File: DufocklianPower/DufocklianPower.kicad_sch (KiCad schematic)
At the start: 84 parts, among them J1 Conn_Receptacle_3P_Protected, J2 ST7796S, Q1 NMOS, Q2 NMOS, SW1 RST, SW2 BOOT, T1 Transformer_1P_1S, U2 LM5164DDA, U3 OPA388, U4 AD5282, U5 MCP4725, U6 ESP32-S3-WROOM-1, U7 INA228

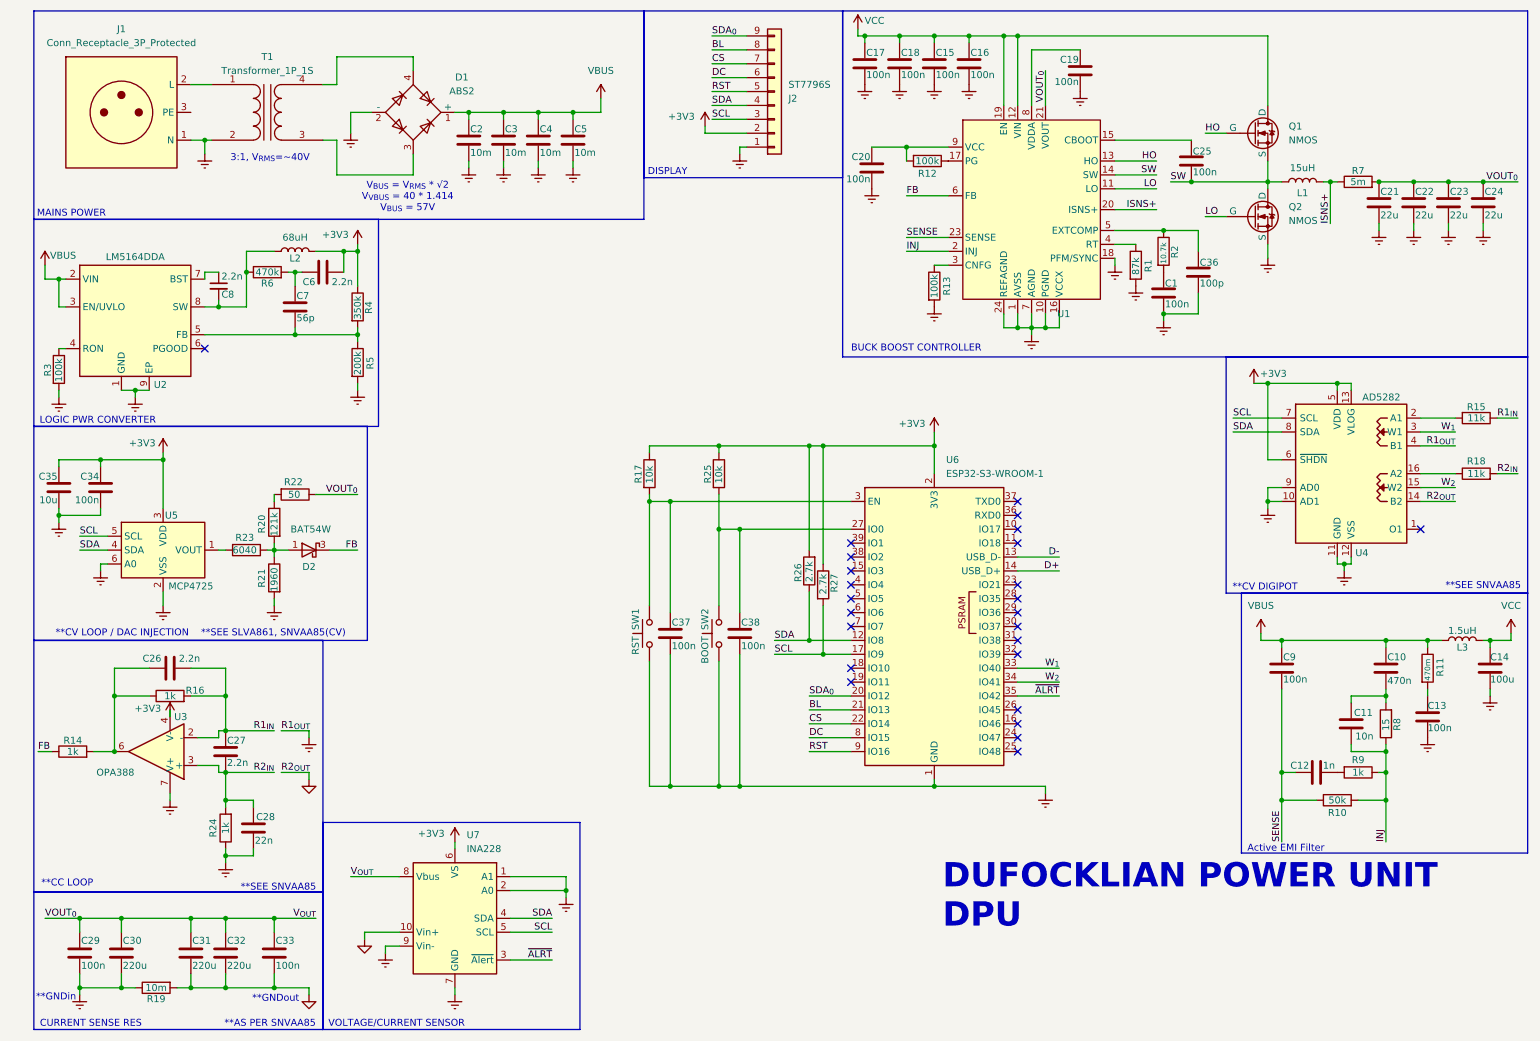
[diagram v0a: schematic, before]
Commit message: finish pcb
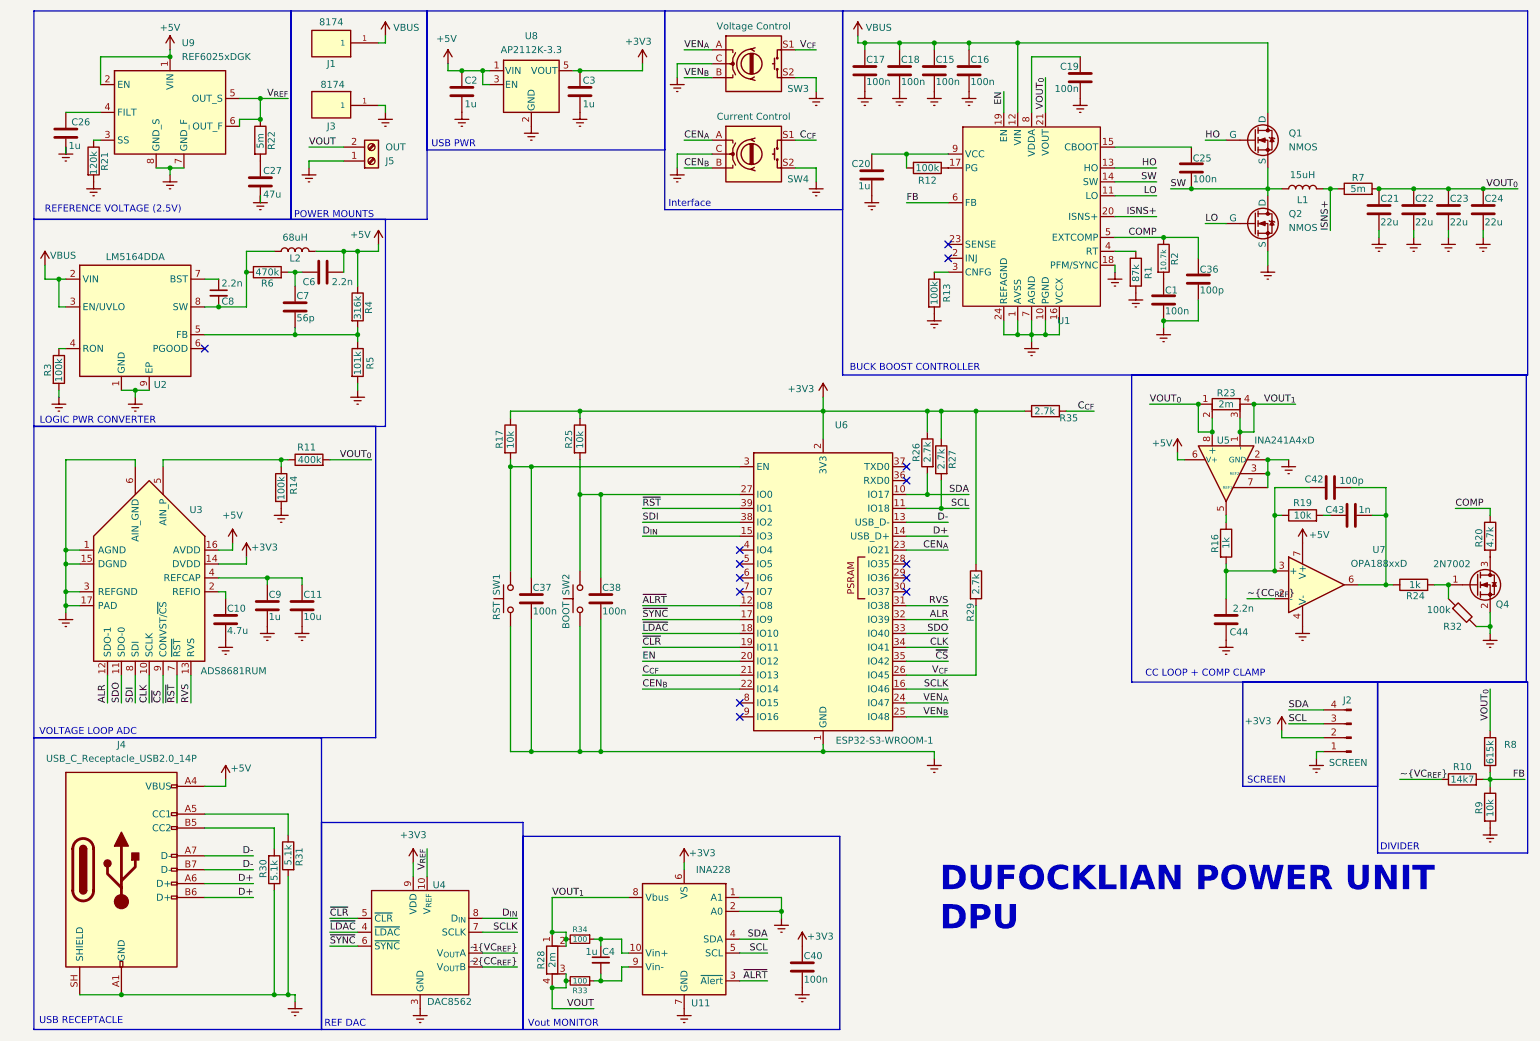
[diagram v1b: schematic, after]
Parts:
- removed C12: 1n, symbol Device:C
- removed C13, C29, C33, C34: 100n, symbol Device:C
- removed C14: 100u, symbol Device:C
- removed C28: 22n, symbol Device:C
- removed C30, C31, C32: 220u, symbol Device:C
- removed C35: 10u, symbol Device:C
- removed C4, C5: 10m, symbol Device:C
- removed D1: ABS2, Diode_SMD:Diode_Bridge_Diotec_ABS, symbol Diode_Bridge:ABS2
- removed D2: BAT54W, Package_TO_SOT_SMD:SOT-323_SC-70, symbol Diode:BAT54W
- removed J1: Conn_Receptacle_3P_Protected, symbol Connector:Conn_Receptacle_3P_Protected
- removed J2: ST7796S, symbol Connector_Generic:Conn_01x09
- removed L3: 1.5uH, symbol Device:L
- removed R15, R18: 11k, symbol Device:R
- removed R23: 6040, symbol Device:R
- removed T1: Transformer_1P_1S, symbol Device:Transformer_1P_1S
- removed U3: OPA388, Package_SO:SOIC-8_3.9x4.9mm_P1.27mm, symbol Amplifier_Operational:OPA333xxD
- removed U4: AD5282, Package_SO:TSSOP-16_4.4x5mm_P0.65mm, symbol Potentiometer_Digital:AD5282
- removed U5: MCP4725, Package_TO_SOT_SMD:SOT-23-6, symbol Analog_DAC:MCP4725xxx-xCH
- removed U7: INA228, Package_SO:TSSOP-10_3x3mm_P0.5mm, symbol Sensor_Energy:INA228
- added C4: 1u, Capacitor_SMD:C_0805_2012Metric, symbol Device:C_Small
- added C40: 100n, Capacitor_SMD:C_0805_2012Metric, symbol Device:C
- added C42: 100p, Capacitor_SMD:C_0805_2012Metric, symbol Device:C
- added C43: 1n, Capacitor_SMD:C_0805_2012Metric, symbol Device:C
- added C44: 2.2n, Capacitor_SMD:C_0805_2012Metric, symbol Device:C
- added J1, J3: 8174, Library:KEYSTONE_8174, symbol dufocklpwr:8174
- added J2: SCREEN, Connector_PinHeader_2.54mm:PinHeader_1x04_P2.54mm_Vertical, symbol Connector:Conn_01x04_Pin
- added J4: USB_C_Receptacle_USB2.0_14P, Connector_USB:USB_C_Receptacle_GCT_USB4105-xx-A_16P_TopMnt_Horizontal, symbol Connector:USB_C_Receptacle_USB2.0_14P
- added J5: OUT, Connector_AMASS:AMASS_XT60PW-M_1x02_P7.20mm_Horizontal, symbol Connector:Screw_Terminal_01x02
- added Q4: 2N7002, Package_TO_SOT_SMD:SOT-23, symbol Transistor_FET:2N7002
- added R23, R28: 2m, Library:FC4L90_OHM, symbol Device:R_Shunt
- added R29, R35: 2.7k, Resistor_SMD:R_0603_1608Metric, symbol Device:R
- added R30, R31: 5.1k, Resistor_SMD:R_0603_1608Metric, symbol Device:R
- added R32: 100k, Resistor_SMD:R_0603_1608Metric, symbol Device:R_45deg
- added R33, R34: 100, Resistor_SMD:R_0603_1608Metric, symbol Device:R_Small
- added SW3: Voltage Control, Rotary_Encoder:RotaryEncoder_Alps_EC11E-Switch_Vertical_H20mm, symbol Device:RotaryEncoder_Switch
- added SW4: Current Control, Rotary_Encoder:RotaryEncoder_Alps_EC11E-Switch_Vertical_H20mm, symbol Device:RotaryEncoder_Switch
- added U11: INA228, Package_SO:TSSOP-10_3x3mm_P0.5mm, symbol Sensor_Energy:INA228
- added U3: ADS8681RUM, Package_DFN_QFN:QFN-16-1EP_4x4mm_P0.65mm_EP2.7x2.7mm, symbol Analog_ADC:ADS8681RUM
- added U4: DAC8562, Package_SO:TSSOP-10_3x3mm_P0.5mm, symbol dufocklpwr:DAC8562
- added U5: INA241A4xD, Package_SO:SOIC-8_3.9x4.9mm_P1.27mm, symbol Amplifier_Current:INA241A4xD
- added U7: OPA188xxD, Package_SO:SOIC-8_3.9x4.9mm_P1.27mm, symbol Amplifier_Operational:OPA188xxD
- added U8: AP2112K-3.3, Package_TO_SOT_SMD:SOT-23-5, symbol Regulator_Linear:AP2112K-3.3
- added U9: REF6025xDGK, Package_SO:VSSOP-8_3x3mm_P0.65mm, symbol Reference_Voltage:REF6025xDGK
- C1, C19, C25, C36, C37, C38, C6, C7, C8: footprint (none) -> Capacitor_SMD:C_0805_2012Metric
- C10: value 470n -> 4.7u; footprint (none) -> Capacitor_SMD:C_0805_2012Metric
- C11: value 10n -> 10u; footprint (none) -> Capacitor_SMD:C_0805_2012Metric
- C15, C16, C17, C18, C21, C22, C23, C24: footprint (none) -> Capacitor_SMD:C_1210_3225Metric
- C2, C3: value 10m -> 1u; footprint (none) -> Capacitor_SMD:C_0805_2012Metric
- C20, C9: value 100n -> 1u; footprint (none) -> Capacitor_SMD:C_0805_2012Metric
- C26: value 2.2n -> 1u; footprint (none) -> Capacitor_SMD:C_0805_2012Metric
- C27: value 2.2n -> 47u; footprint (none) -> Capacitor_SMD:C_0805_2012Metric
- L1: footprint (none) -> Library:IND_SER2915H-223KL
- L2: footprint (none) -> Library:IND_BOURNS_SRR1260
- Q1, Q2: footprint (none) -> Library:TRANS_BSC027N10NS5ATMA1
- R1, R12, R13, R16, R17, R2, R24, R25, R26, R27, R3, R6: footprint (none) -> Resistor_SMD:R_0603_1608Metric
- R10: value 50k -> 14k7; footprint (none) -> Resistor_SMD:R_0603_1608Metric
- R11: value 470m -> 400k; footprint (none) -> Resistor_SMD:R_0603_1608Metric
- R14: value 1k -> 100k; footprint (none) -> Resistor_SMD:R_0603_1608Metric
- R19: value 10m -> 10k; footprint (none) -> Resistor_SMD:R_0603_1608Metric
- R20: value 121k -> 4.7k; footprint (none) -> Resistor_SMD:R_0603_1608Metric
- R21: value 1960 -> 120k; footprint (none) -> Resistor_SMD:R_0603_1608Metric
- R22: value 50 -> 5m; footprint (none) -> Resistor_SMD:R_0603_1608Metric
- R4: value 350k -> 316k; footprint (none) -> Resistor_SMD:R_0603_1608Metric
- R5: value 200k -> 101k; footprint (none) -> Resistor_SMD:R_0603_1608Metric
- R7: footprint (none) -> Resistor_SMD:R_2512_6332Metric
- R8: value 15 -> 615k; footprint (none) -> Resistor_SMD:R_0603_1608Metric
- R9: value 1k -> 10k; footprint (none) -> Resistor_SMD:R_0603_1608Metric
- SW1, SW2: footprint (none) -> Button_Switch_SMD:SW_Push_1P1T-SH_NO_CK_KMR2xxG
- U1: footprint (none) -> Library:VQFN24_RGY_TEX
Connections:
- net +3V3: now also C3.1, R26.1, C40.1, J2.2 (Pin_2), R29.1, R35.1, U11.6 (VS), U3.14 (DVDD), U4.9 (VDD), U8.5 (VOUT); no longer C6.2, L2.2, R26.2, R4.1
- net D+: now also J4.A6 (D+), J4.B6 (D+)
- net D-: now also J4.A7 (D-), J4.B7 (D-)
- net FB: now also R10.2, R8.2, R9.1; no longer R14.1
- net GND: now also C1.2, C10.1, C11.1, C15.2, C16.2, C17.2, C18.2, C19.2, C2.2, C20.2, C21.2, C22.2, C23.2, C24.2, C26.2, C27.2, C3.2, C36.2, C37.2, C38.2, C9.1, Q2.3 (S), R1.2, R13.2, R14.2, R21.2, R3.2, R5.2, R9.2, SW1.1, SW2.1, U1.1 (AVSS), U1.10 (PGND), U1.16 (VCCX), U1.18 (PFM/SYNC), U1.24 (REFAGND), U1.25 (GND), U1.7 (AGND), U2.1 (GND), U2.9 (EP), U6.1 (GND), U6.40 (GND), U6.41 (GND), C40.2, C44.1, J2.1 (Pin_1), J3.1, J3.2 (1__1), J3.3 (1__2), J3.4 (1__3), J4.A1 (GND), J4.A12 (GND), J4.B1 (GND), J4.B12 (GND), J4.SH (SHIELD), J5.1 (Pin_1), Q4.2 (S), R30.1, R31.2, R32.2, SW3.C, SW3.S2, SW4.C, SW4.S2, U11.1 (A1), U11.2 (A0), U11.7 (GND), U3.1 (AGND), U3.15 (DGND), U3.17 (PAD), U3.3 (REFGND), U3.6 (AIN_GND), U4.3 (GND), U5.2 (GND), U5.3 (REF2), U5.4 (GND), U5.7 (REF1), U7.4 (V-), U8.2 (GND), U9.7 (GND_F), U9.8 (GND_S); no longer R19.2
- net SCL: now also U6.11 (IO18), J2.3 (Pin_3), U11.5 (SCL); no longer U6.17 (IO9)
- net SDA: now also R26.2, U6.10 (IO17), J2.4 (Pin_4), U11.4 (SDA); no longer R26.1, U6.12 (IO8)
- net VBUS: now also C15.1, C16.1, C17.1, C18.1, Q1.1 (D), U1.12 (VIN), J1.1, J1.2 (1__1), J1.3 (1__2), J1.4 (1__3); no longer C10.1, C2.1, C3.1, C9.1, R11.1
- net VOUT_{0}: now also R11.2, R8.1, R23.1, R23.2, U5.8 (+); no longer R22.1
- net ~{ALRT}: now also U6.12 (IO8), U11.3 (~{Alert}); no longer U6.35 (IO42)
- net at R22.2: now also C27.1; no longer R20.1
- net at R20.2: now also Q4.3 (D); no longer R21.1
- net COMP: now reaches C36.1, R2.1, U1.5 (EXTCOMP)
- net COMP: now also R20.1
- net D_{IN}: now reaches U6.15 (IO3)
- net D_{IN}: now also U4.8 (D_{IN})
- net SCLK: now reaches U6.16 (IO46)
- net SCLK: now also U4.7 (SCLK)
- net ~{LDAC}: now reaches U6.18 (IO10)
- net ~{LDAC}: now also U4.4 (~{LDAC})
- net ~{CLR}: now reaches U6.19 (IO11)
- net ~{CLR}: now also U4.5 (~{CLR})
- net CEN_{A}: now reaches U6.23 (IO21)
- net CEN_{A}: now also SW4.A
- net VEN_{A}: now reaches U6.24 (IO47)
- net VEN_{A}: now also SW3.A
- net VEN_{B}: now reaches U6.25 (IO48)
- net VEN_{B}: now also SW3.B
- net V_{CF}: now reaches U6.26 (IO45)
- net V_{CF}: now also R29.2, SW3.S1
- net RVS: now reaches U6.31 (IO38)
- net RVS: now also U3.13 (RVS)
- net ALR: now reaches U6.32 (IO39)
- net ALR: now also U3.12 (SDO-1)
- net SDI: now reaches U6.38 (IO2)
- net SDI: now also U3.8 (SDI)
- net ~{RST}: now reaches U6.39 (IO1)
- net ~{RST}: now also U3.7 (~{RST})
- net BL renamed C_{CF}
- net C_{CF}: now also R35.2, SW4.S1
- net CS renamed CEN_{B}
- net CEN_{B}: now also SW4.B
- net DC: no longer names the net of U6.8 (IO15)
- removed net GNDREF: C1.2, C15.2, C16.2, C17.2, C18.2, C19.2, C2.2, C20.2, C21.2, C22.2, C23.2, C24.2, C3.2, C36.2, C37.2, C38.2, Q2.3 (S), R1.2, R13.2, R19.1, R21.2, R24.1, R3.2, R5.2, SW1.1, SW2.1, U1.1 (AVSS), U1.10 (PGND), U1.16 (VCCX), U1.18 (PFM/SYNC), U1.24 (REFAGND), U1.7 (AGND), U2.1 (GND), U2.9 (EP), U6.1 (GND), U6.40 (GND), U6.41 (GND)
- removed net INJ: C11.2, R10.2, R8.1, R9.1, U1.2 (INJ)
- removed net R1_{IN}: C26.2, C27.1, R16.2
- net R2_{IN}: no longer names the net of R24.2
- net R2_{IN}: now also Q4.1 (G), R32.1; no longer C27.2
- net RST: no longer names the net of U6.9 (IO16)
- net SDA_{0} renamed EN
- net EN: now also U1.19 (EN)
- removed net SENSE: C9.2, R10.1, U1.23 (SENSE)
- removed net VCC: C15.1, C16.1, C17.1, C18.1, Q1.1 (D), U1.12 (VIN), U1.19 (EN)
- net W_{1} renamed SDO
- net SDO: now also U3.11 (SDO-0)
- net W_{2} renamed CLK
- net CLK: now also U3.10 (SCLK)
- new net: C4.1, R34.1, U11.10 (Vin+)
- new net: C10.2, U3.2 (REFIO)
- new net: C4.2, R33.1, U11.9 (Vin-)
- new net: C42.1, C44.2, R16.2, R19.1, U7.3 (+)
- new net: C42.2, C43.2, R24.1, U7.6
- new net: J4.B5 (CC2), R30.2
- new net: R11.1, R14.1, U3.5 (AIN_P)
- new net: C43.1, R19.2
- new net: C11.2, C9.2, U3.4 (REFCAP)
- new net: C26.1, U9.4 (FILT)
- new net: J4.A5 (CC1), R31.1
- new net: R16.1, U5.5
- new net: R21.1, U9.3 (SS)
- new net +5V: C2.1, C6.2, J4.A4 (VBUS), J4.A9 (VBUS), J4.B4 (VBUS), J4.B9 (VBUS), L2.2, R4.1, U3.16 (AVDD), U5.6 (V+), U7.7 (V+), U8.1 (VIN), U8.3 (EN), U9.1 (VIN), U9.2 (EN)
- new net VOUT: J5.2 (Pin_2), R28.3, R28.4, R33.2
- new net VOUT_{1}: R23.3, R23.4, R28.1, R28.2, R34.2, U11.8 (Vbus), U5.1 (-)
- new net V_{REF}: R22.1, U4.10 (V_{REF}), U9.5 (OUT_S), U9.6 (OUT_F)
- new net ~{CC_{REF}}: U4.2 (V_{OUT}B), U7.2 (-)
- new net ~{CS}: U3.9 (CONVST/~{CS}), U6.35 (IO42)
- new net ~{SYNC}: U4.6 (~{SYNC}), U6.17 (IO9)
- new net ~{VC_{REF}}: R10.1, U4.1 (V_{OUT}A)
- no-connect marks 25 -> 14
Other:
- note added: "CC LOOP + COMP CLAMP"
- note added: "DIVIDER"
- note added: "Interface"
- note added: "POWER MOUNTS"
- note added: "REF DAC"
- note added: "REFERENCE VOLTAGE (2.5V)"
- note added: "SCREEN"
- note added: "USB PWR"
- note added: "USB RECEPTACLE"
- note added: "VOLTAGE LOOP ADC"
- note added: "Vout MONITOR"
- note removed: "**AS PER SNVAA85"
- note removed: "**CC LOOP"
- note removed: "**CV DIGIPOT"
- note removed: "**CV LOOP / DAC INJECTION **SEE SLVA861, SNVAA85(CV)"
- note removed: "**GNDin"
- note removed: "**GNDout"
- note removed: "**SEE SNVAA85"
- note removed: "3:1, V_{RMS}=~40V"
- note removed: "Active EMI Filter"
- note removed: "CURRENT SENSE RES"
- note removed: "DISPLAY"
- note removed: "MAINS POWER"
- note removed: "VOLTAGE/CURRENT SENSOR"
- note removed: "V_{BUS} = V_{RMS} * √2 V_{VBUS} = 40 * 1.414 V_{BUS} = 57V"
- moved on the sheet: C1, C15, C16, C17, C18, C19, C20, C21, C22, C23, C24, C25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
